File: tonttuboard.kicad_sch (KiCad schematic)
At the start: 45 parts, among them U3 ICM-40609-D, U4 BMP388, U5 W25Q256JVFIQT, U6 MMC5983MA, U9 Teensy 4.0

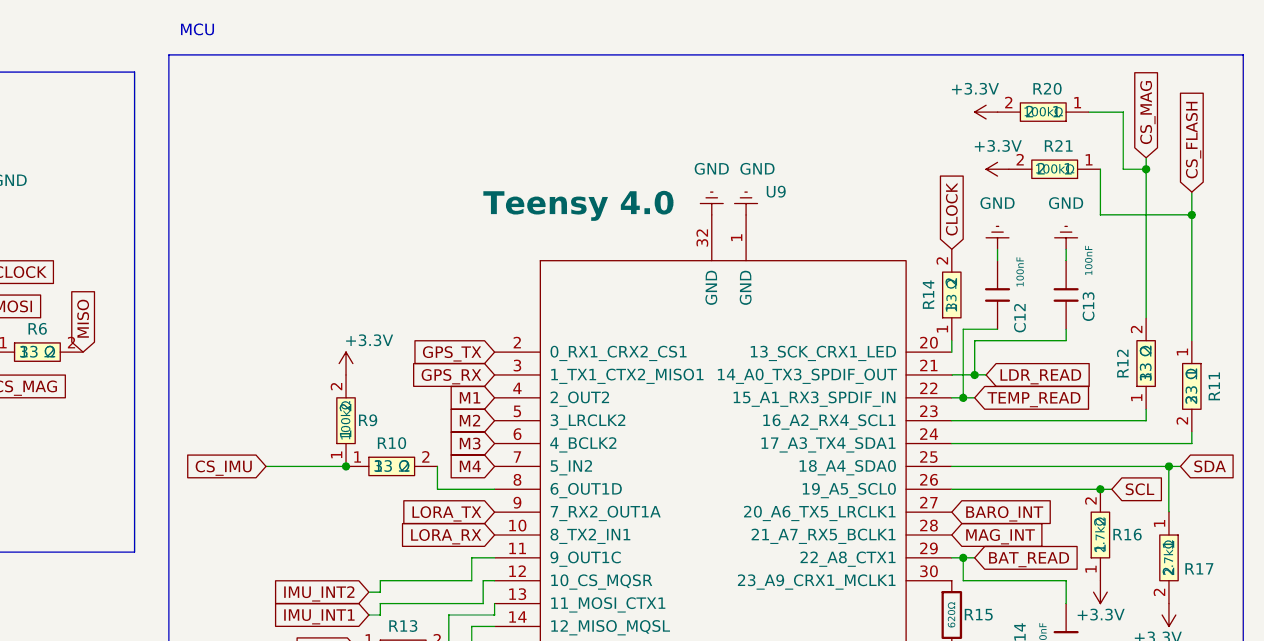
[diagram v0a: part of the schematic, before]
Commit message: Added gnd vias and decorated
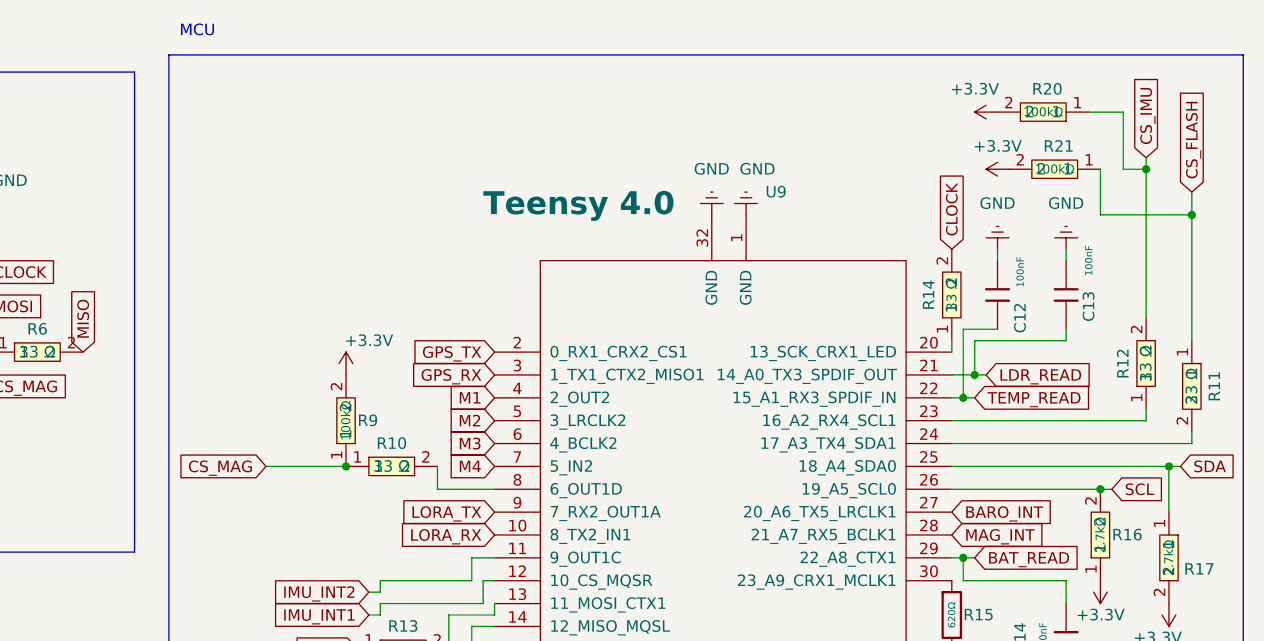
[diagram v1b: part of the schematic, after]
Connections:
- net CS_IMU: now also R12.2, R20.1; no longer R10.1, R9.1
- net CS_MAG: now also R10.1, R9.1; no longer R12.2, R20.1
